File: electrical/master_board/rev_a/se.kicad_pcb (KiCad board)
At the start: 2 copper layers, 64.7 x 45 mm, 0 parts

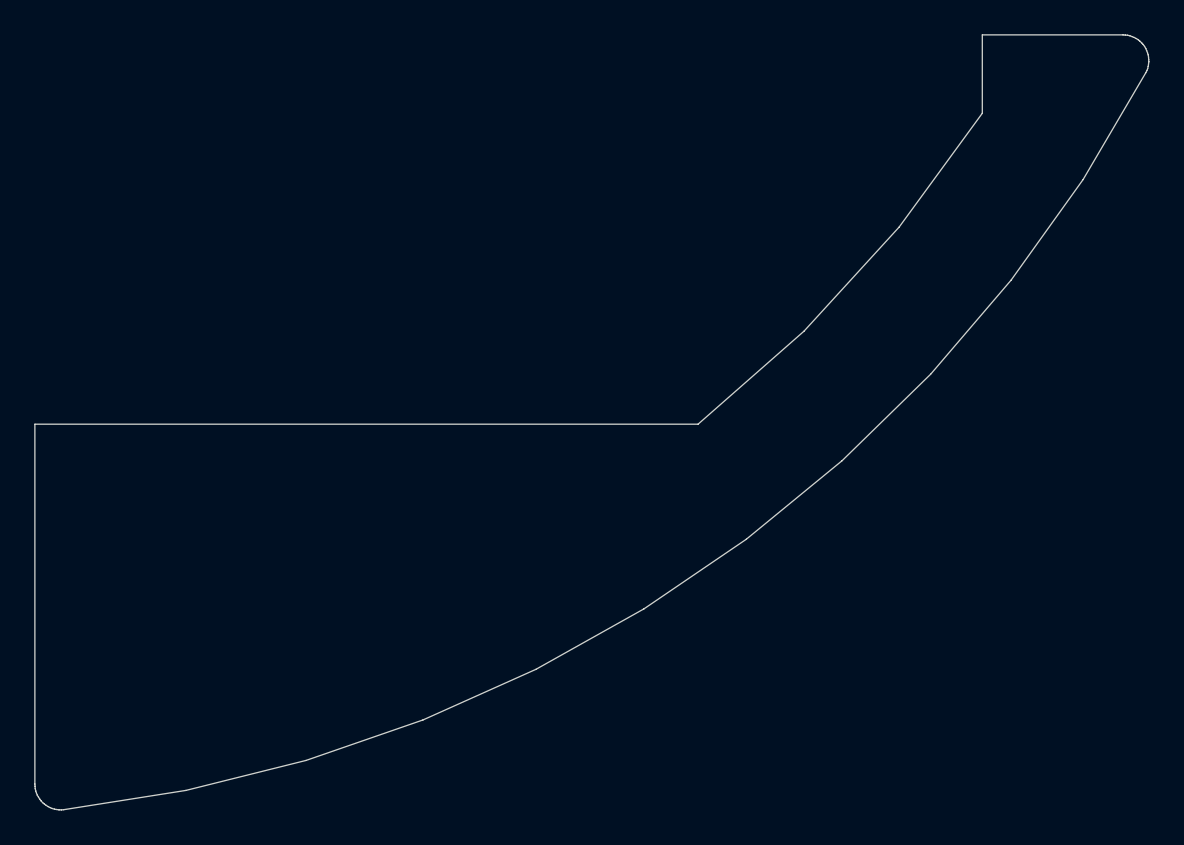
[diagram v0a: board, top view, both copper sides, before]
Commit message: Finally have everything fitting together.
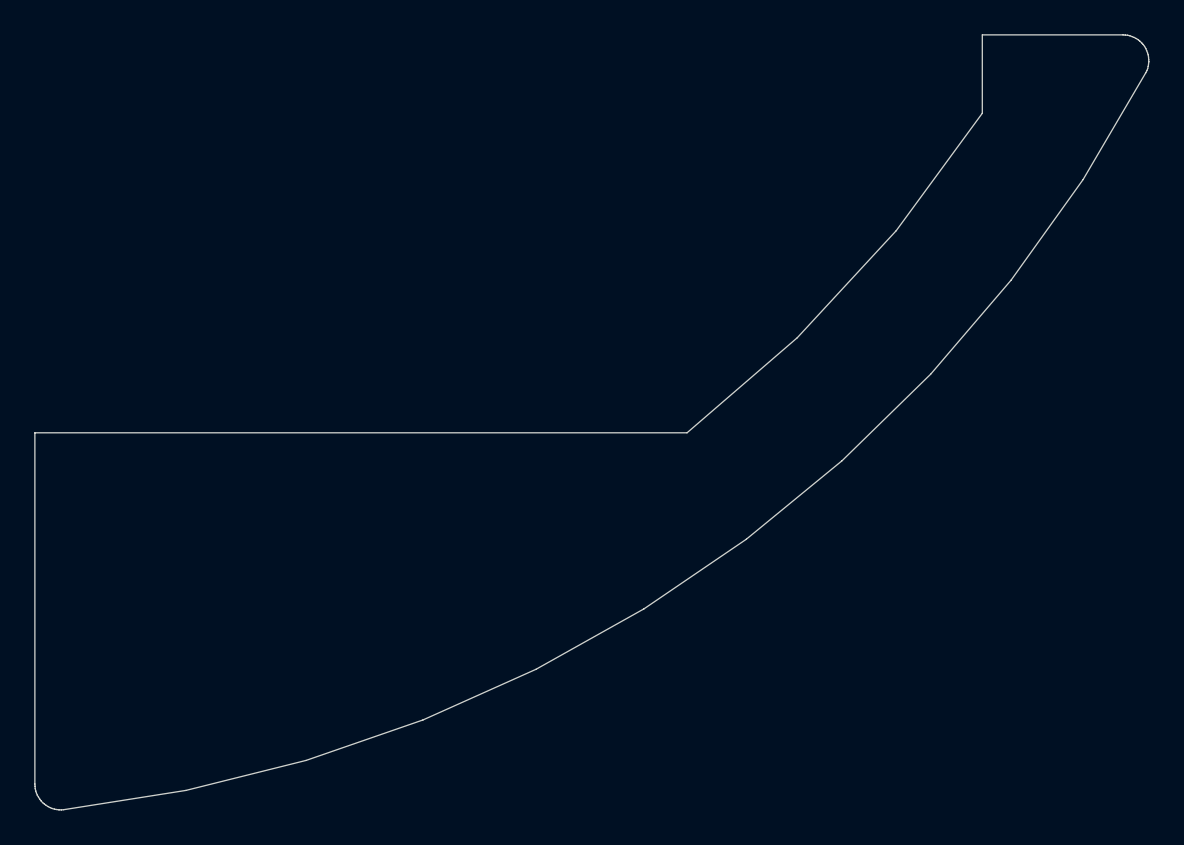
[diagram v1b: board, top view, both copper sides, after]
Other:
- outline, holes or cut-outs redrawn
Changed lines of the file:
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@@
     (uvia_drill 0.1)
   )
-  (gr_line (start 107.5 158.6) (end 107.5 179.49) (layer Edge.Cuts) (width 0.05))
+  (gr_line (start 107.5 159.1) (end 107.5 179.49) (layer Edge.Cuts) (width 0.05))
   (gr_line (start 107.5 179.49) (end 107.51 179.62) (layer Edge.Cuts) (width 0.05))
   (gr_line (start 107.51 179.62) (end 107.52 179.76) (layer Edge.Cuts) (width 0.05))
@@
   (gr_line (start 170.67 136) (end 162.5 136) (layer Edge.Cuts) (width 0.05))
   (gr_line (start 162.5 136) (end 162.5 140.55) (layer Edge.Cuts) (width 0.05))
-  (gr_line (start 162.5 140.55) (end 157.67 147.16) (layer Edge.Cuts) (width 0.05))
-  (gr_line (start 157.67 147.16) (end 152.15 153.2) (layer Edge.Cuts) (width 0.05))
-  (gr_line (start 152.15 153.2) (end 146 158.6) (layer Edge.Cuts) (width 0.05))
-  (gr_line (start 146 158.6) (end 107.5 158.6) (layer Edge.Cuts) (width 0.05))
+  (gr_line (start 162.5 140.55) (end 157.5 147.37) (layer Edge.Cuts) (width 0.05))
+  (gr_line (start 157.5 147.37) (end 151.76 153.58) (layer Edge.Cuts) (width 0.05))
+  (gr_line (start 151.76 153.58) (end 145.36 159.1) (layer Edge.Cuts) (width 0.05))
+  (gr_line (start 145.36 159.1) (end 107.5 159.1) (layer Edge.Cuts) (width 0.05))
 )
